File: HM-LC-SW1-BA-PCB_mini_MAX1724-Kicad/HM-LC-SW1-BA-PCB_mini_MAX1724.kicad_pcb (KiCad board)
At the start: 2 copper layers, 20 x 40 mm, 30 parts, among them IC1 ATMEGA328P-A, IC2 CC1101, J1 Conn_01x03_Female, J2 Conn_01x03_Female, P3 ANT, P4 ISP Bottom, P5 ISP Top, Q1 IRLML2803, SW1 Reset, SW2 Config, U1 MAX1724, Y1 Crystal

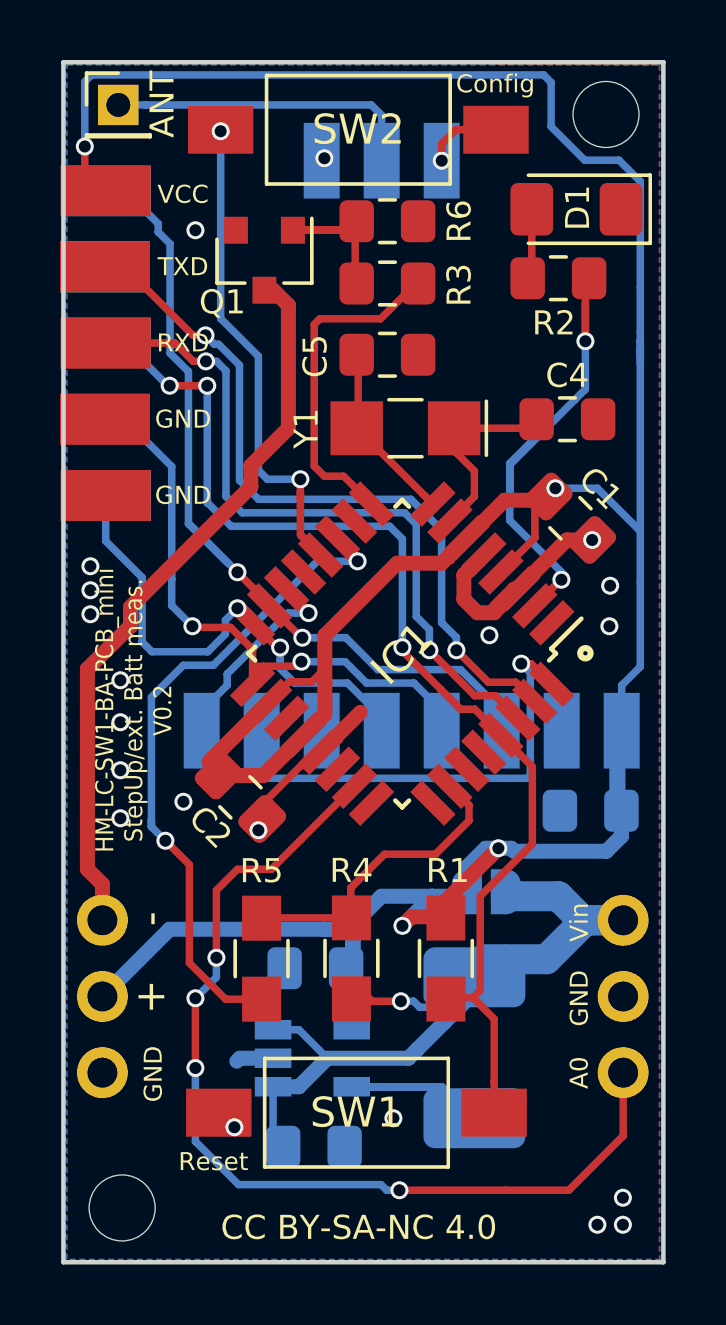
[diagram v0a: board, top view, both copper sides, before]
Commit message: update V0.2
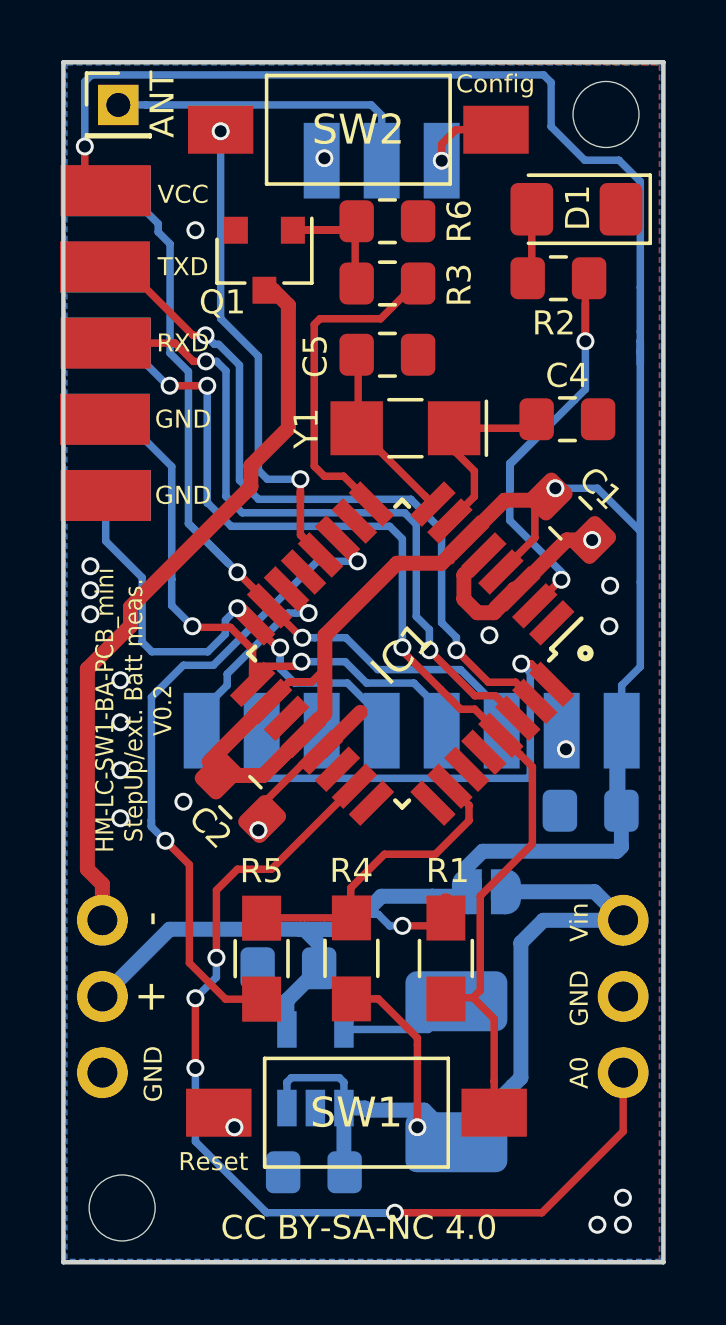
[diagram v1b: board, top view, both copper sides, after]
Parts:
- moved C6 0.90 mm to (177.5, 115.2)
- moved C7 0.85 mm to (178.3, 122.0), turned to 180 degrees
- moved L1 0.61 mm to (183.1, 118.2), turned to 90 degrees
- moved U1 0.36 mm to (178.4, 118.5), turned to 90 degrees
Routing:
- net Net-(L1-Pad2): track 7.65 -> 4.14 mm
- net VCC: track 124.4 -> 121.4 mm, vias 4 -> 3
- net GND: track 20.2 -> 17.9 mm
- net /A0: track 32.9 -> 34.5 mm
- net /Vin: track 32.6 -> 33.3 mm

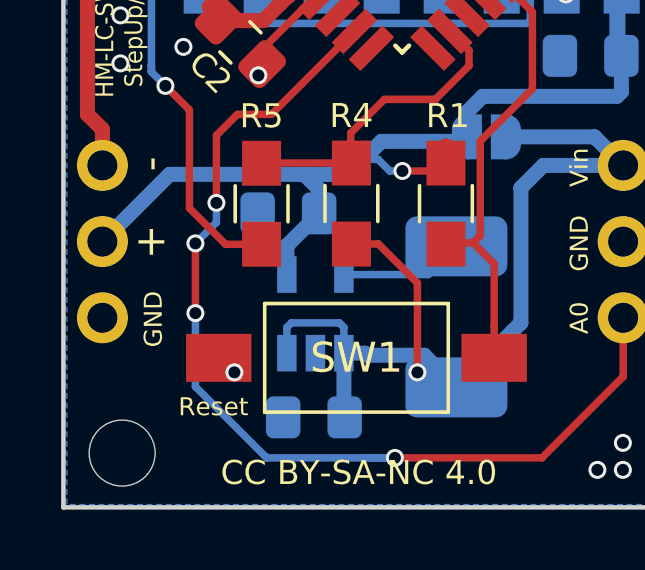
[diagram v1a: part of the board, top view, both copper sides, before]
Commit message: update V0.2
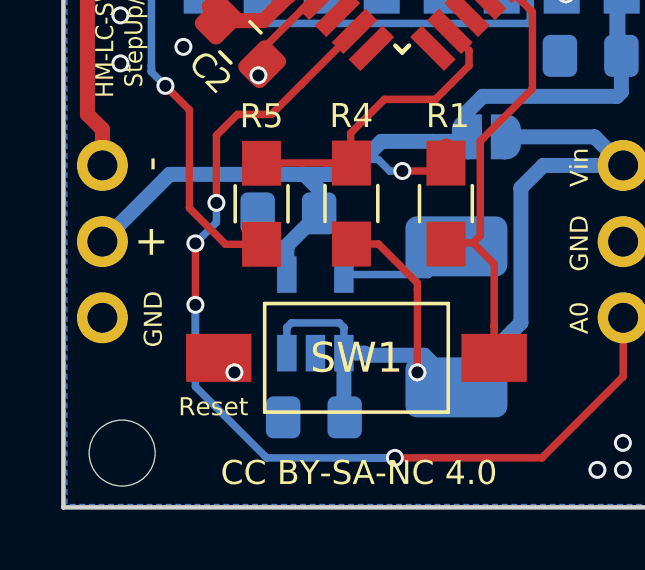
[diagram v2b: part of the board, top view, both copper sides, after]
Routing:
- net /A0: track 34.5 -> 36.7 mm
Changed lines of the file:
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@@
     (thickness 1.6)
     (drawings 23)
-    (tracks 440)
+    (tracks 442)
     (zones 0)
     (modules 30)
@@
   (gr_line (start 190 85) (end 190 125) (angle 90) (layer Edge.Cuts) (width 0.15))
   (gr_line (start 170 85) (end 190 85) (angle 90) (layer Edge.Cuts) (width 0.15))
-  (via (at 186.75 107.9) (size 0.6) (drill 0.4) (layers F.Cu B.Cu) (net 2))
-  (via (at 181.8 120.5) (size 0.6) (drill 0.4) (layers F.Cu B.Cu) (net 22))
   (segment (start 189.23 88.9762) (end 189.23 92.5068) (width 0.25) (layer B.Cu) (net 1))
   (segment (start 189.23 95.061738) (end 189.23 94.6404) (width 0.25) (layer B.Cu) (net 1))
@@
   (segment (start 180.875736 113.7864) (end 180.489336 113.4) (width 0.25) (layer B.Cu) (net 1))
   (segment (start 181.3 113.7864) (end 180.875736 113.7864) (width 0.25) (layer B.Cu) (net 1))
+  (segment (start 177.45 116.275) (end 178.525 115.2) (width 0.5) (layer B.Cu) (net 1))
+  (segment (start 177.45 117.24) (end 177.45 116.275) (width 0.5) (layer B.Cu) (net 1))
+  (segment (start 178.025 113.9) (end 177.9 113.9) (width 0.5) (layer B.Cu) (net 1))
+  (segment (start 178.525 114.4) (end 178.025 113.9) (width 0.5) (layer B.Cu) (net 1))
+  (segment (start 178.525 115.2) (end 178.525 114.4) (width 0.5) (layer B.Cu) (net 1))
+  (segment (start 178.7 113.9) (end 177.9 113.9) (width 0.5) (layer B.Cu) (net 1))
+  (segment (start 177.9 113.9) (end 177 113.9) (width 0.5) (layer B.Cu) (net 1))
+  (via (at 186.75 107.9) (size 0.6) (drill 0.4) (layers F.Cu B.Cu) (net 2))
   (via (at 176.5 110.6) (size 0.6) (drill 0.4) (layers F.Cu B.Cu) (net 2))
   (via (at 178.7 88.2) (size 0.6) (drill 0.4) (layers F.Cu B.Cu) (net 2))
@@
   (via (at 188.225 102.45) (size 0.6) (drill 0.4) (layers F.Cu B.Cu) (net 2))
   (via (at 188.2 103.8) (size 0.6) (drill 0.4) (layers F.Cu B.Cu) (net 2))
-  (segment (start 177.45 116.275) (end 178.525 115.2) (width 0.5) (layer B.Cu) (net 1))
-  (segment (start 177.45 117.24) (end 177.45 116.275) (width 0.5) (layer B.Cu) (net 1))
-  (segment (start 178.025 113.9) (end 177.9 113.9) (width 0.5) (layer B.Cu) (net 1))
-  (segment (start 178.525 114.4) (end 178.025 113.9) (width 0.5) (layer B.Cu) (net 1))
-  (segment (start 178.525 115.2) (end 178.525 114.4) (width 0.5) (layer B.Cu) (net 1))
-  (segment (start 178.7 113.9) (end 177.9 113.9) (width 0.5) (layer B.Cu) (net 1))
-  (segment (start 177.9 113.9) (end 177 113.9) (width 0.5) (layer B.Cu) (net 1))
   (segment (start 186.699027 102.1334) (end 185.711917 103.12051) (width 0.25) (layer F.Cu) (net 3))
   (via (at 186.6 102.25) (size 0.6) (drill 0.4) (layers F.Cu B.Cu) (net 3))
@@
   (segment (start 179.70151 109.130917) (end 177.933614 110.898813) (width 0.25) (layer F.Cu) (net 15))
   (via (at 174.4 116.2) (size 0.6) (drill 0.4) (layers F.Cu B.Cu) (net 15))
-  (via (at 174.4 118.525) (size 0.6) (drill 0.4) (layers F.Cu B.Cu) (net 15))
+  (via (at 174.4 118.25) (size 0.6) (drill 0.4) (layers F.Cu B.Cu) (net 15))
   (segment (start 176.932427 111.9) (end 177.933614 110.898813) (width 0.25) (layer F.Cu) (net 15))
   (segment (start 175.8 111.9) (end 176.932427 111.9) (width 0.25) (layer F.Cu) (net 15))
@@
   (segment (start 175.1 115.5) (end 174.4 116.2) (width 0.25) (layer B.Cu) (net 15))
   (segment (start 175.1 114.85) (end 175.1 115.5) (width 0.25) (layer B.Cu) (net 15))
-  (segment (start 174.4 118.525) (end 174.4 116.2) (width 0.25) (layer F.Cu) (net 15))
-  (segment (start 174.4 120.975) (end 174.4 118.525) (width 0.25) (layer B.Cu) (net 15))
   (segment (start 176.725 123.3) (end 174.4 120.975) (width 0.25) (layer B.Cu) (net 15))
   (segment (start 180 123.35) (end 181.05 123.35) (width 0.25) (layer B.Cu) (net 15))
@@
   (segment (start 181.05 123.35) (end 185.95 123.35) (width 0.25) (layer F.Cu) (net 15))
   (segment (start 188.6585 120.6415) (end 188.6585 118.6815) (width 0.25) (layer F.Cu) (net 15))
+  (segment (start 174.4 116.2) (end 174.4 118.25) (width 0.25) (layer F.Cu) (net 15))
+  (segment (start 174.4 118.25) (end 174.4 120.8) (width 0.25) (layer B.Cu) (net 15))
+  (segment (start 174.4 120.975) (end 174.4 120.8) (width 0.25) (layer B.Cu) (net 15))
+  (segment (start 174.4 120.8) (end 174.4 118.525) (width 0.25) (layer B.Cu) (net 15))
   (segment (start 179.578 113.5215) (end 176.6151 113.5215) (width 0.25) (layer F.Cu) (net 17))
   (segment (start 176.6151 113.5215) (end 176.6062 113.5304) (width 0.25) (layer F.Cu) (net 17))
@@
   (segment (start 179.825 95.1) (end 179.475 94.75) (width 0.25) (layer F.Cu) (net 19))
   (segment (start 179.825 97.1) (end 179.825 95.1) (width 0.25) (layer F.Cu) (net 19))
+  (via (at 181.8 120.5) (size 0.6) (drill 0.4) (layers F.Cu B.Cu) (net 22))
   (segment (start 184.5 113.05) (end 184.75 112.8) (width 0.25) (layer B.Cu) (net 22))
   (segment (start 179.6565 116.3) (end 179.578 116.2215) (width 0.25) (layer F.Cu) (net 22))
